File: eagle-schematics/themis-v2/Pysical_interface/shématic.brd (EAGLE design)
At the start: 160 x 100 mm, 35 parts, among them IC1 MCP23017SO, SW1 EC12E_SW, SW2 EC12E_SW, SW3 EC12E_SW, SW4 EC12E_SW

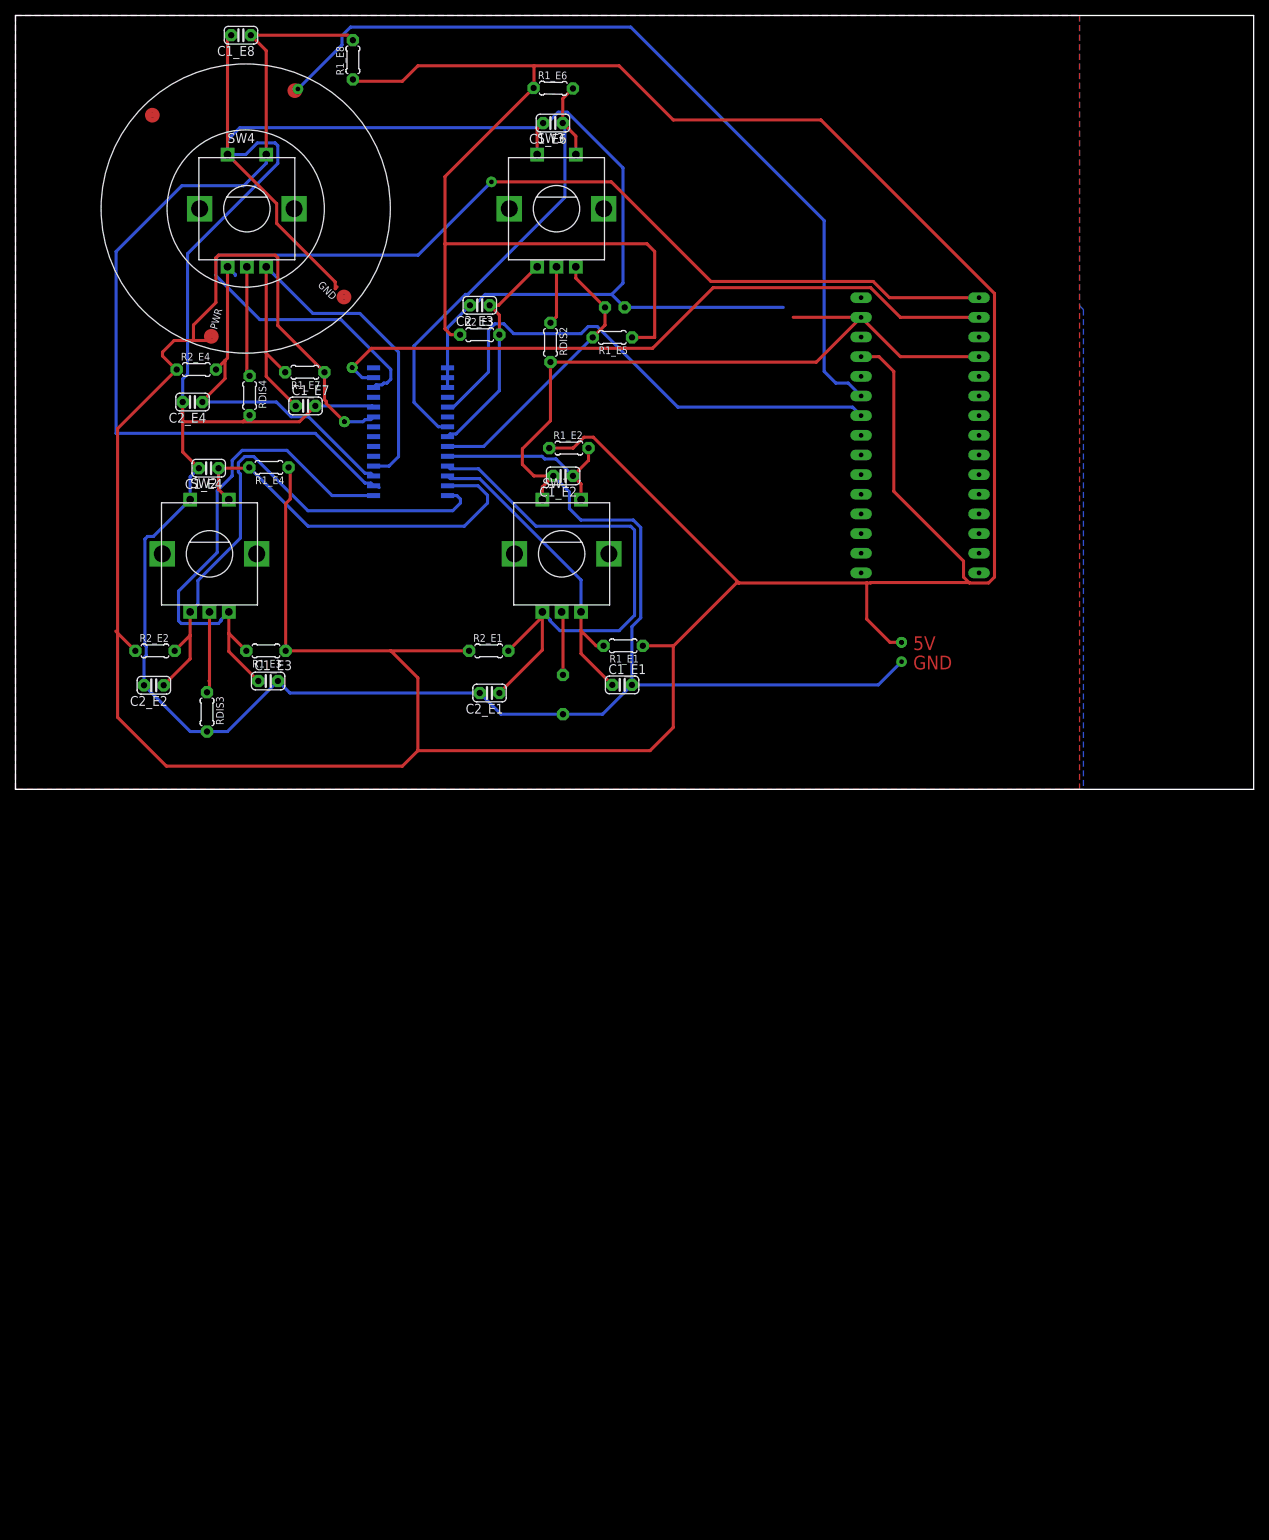
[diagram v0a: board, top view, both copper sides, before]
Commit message: Updated PCB
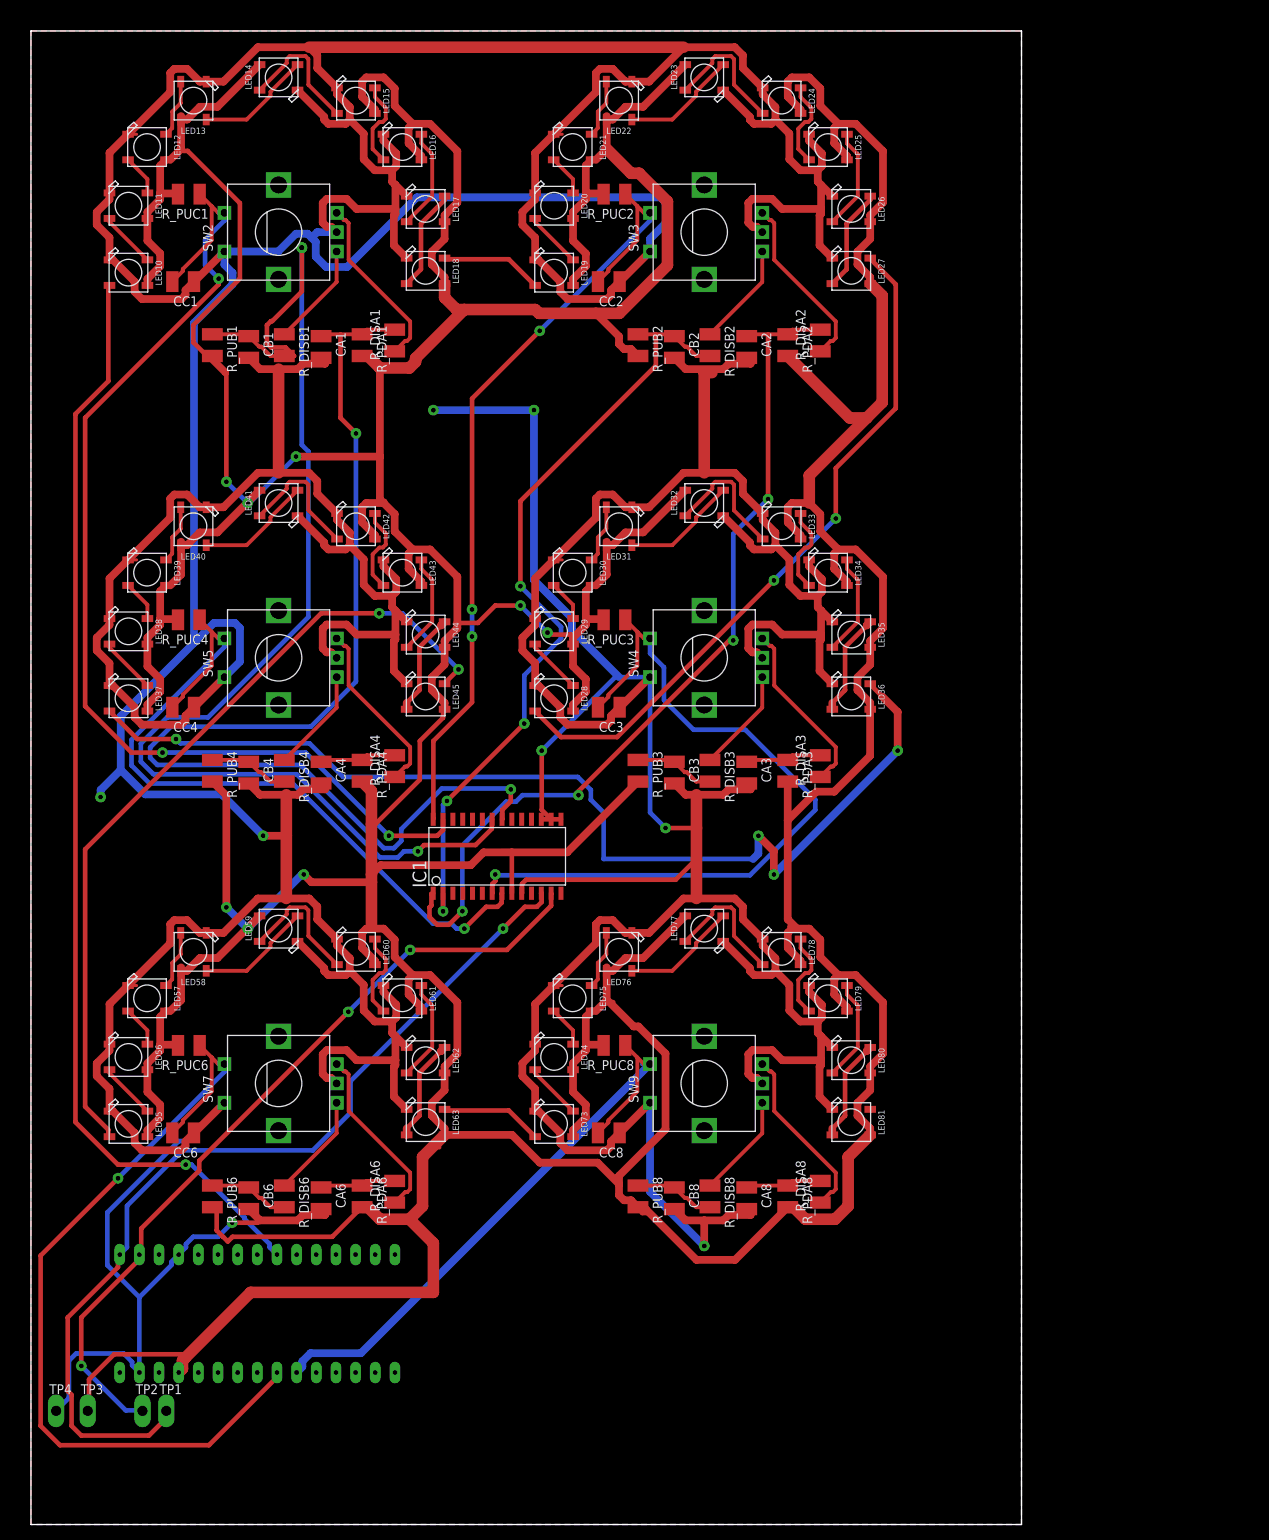
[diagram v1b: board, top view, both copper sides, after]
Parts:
- removed C1_E1, C1_E2, C1_E3, C1_E4, C1_E5, C1_E6, C1_E7, C1_E8, C2_E1, C2_E2, C2_E3, C2_E4: 100n, rcl:C025-024X044
- removed NEOPIXEL1: NEOPIXEL12, Neopixel:NEOPIXEL12
- removed R1_E1, R1_E2, R1_E3, R1_E4, R1_E5, R1_E6, R1_E7, R1_E8, R2_E1, R2_E2, R2_E3, R2_E4: 100k, resistor:0204/5
- removed RDIS1, RDIS2, RDIS3, RDIS4: 1k, resistor:0204/5
- removed SW1: EC12E_SW, switch-alps:ALPS_EC12E_SW
- added CA1, CA2, CA3, CA4, CA6, CA8, CB1, CB2, CB3, CB4, CB6, CB8, CC1, CC2, CC3, CC4, CC6, CC8: 100n, rcl:C1210
- added LED10, LED11, LED12, LED13, LED14, LED15, LED16, LED17, LED18, LED19, LED20, LED21, LED22, LED23, LED24, LED25, LED26, LED27, LED28, LED29, LED30, LED31, LED32, LED33, LED34, LED35, LED36, LED37, LED38, LED39, LED40, LED41, LED42, LED43, LED44, LED45, LED55, LED56, LED57, LED58, LED59, LED60, LED61, LED62, LED63, LED73, LED74, LED75, LED76, LED77, LED78, LED79, LED80, LED81: WS2812B5050, WS2812B:WS2812B
- added R_DISA1, R_DISA2, R_DISA3, R_DISA4, R_DISA6, R_DISA8, R_DISB1, R_DISB2, R_DISB3, R_DISB4, R_DISB6, R_DISB8: 1k, rcl:R1210
- added R_PDA1, R_PDA2, R_PDA3, R_PDA4, R_PDA6, R_PDA8, R_PUB1, R_PUB2, R_PUB3, R_PUB4, R_PUB6, R_PUB8, R_PUC1, R_PUC2, R_PUC3, R_PUC4, R_PUC6, R_PUC8: 100k, rcl:R1210
- added SW5, SW7, SW9: EC12E_SW, switch-alps:ALPS_EC12E_SW
- added TP1, TP2, TP3, TP4: PTR1PAD1-13Y, testpad:P1-13Y
- moved U$2 144.1 mm to (31.2, -75.4), turned to 0 degrees
- moved SW4 82.8 mm to (89.0, 17.0), turned to 90 degrees
- moved IC1 55.2 mm to (61.6, -8.65), flipped to the top, turned to 0 degrees
- moved SW2 42.5 mm to (34.0, 72.0), turned to 90 degrees
- moved SW3 19.3 mm to (89.0, 72.0), turned to 90 degrees
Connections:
- net INTA renamed INTROT_2
- net N$3 renamed INTROT1
- removed net BOUT_1: C1_E6.1, IC1.21, R1_E6.2, SW3.E
- removed net BOUT_2: C1_E2.1, IC1.24, R1_E2.2, SW1.E
- removed net BOUT_3: C1_E4.1, IC1.27, R1_E4.2, SW2.E
- removed net BOUT_4: C1_E8.1, IC1.2, R1_E8.2, SW4.E
- removed net DISCHARGE: RDIS1.1, RDIS2.1, RDIS3.1, RDIS4.1, SW1.C, SW2.C, SW3.C, SW4.C
- removed net EC1_1: C2_E3.1, IC1.22, R2_E3.2, SW3.A
- removed net EC1_2: C1_E5.1, IC1.23, R1_E5.2, SW3.B
- removed net EC2_1: C2_E1.1, IC1.25, R2_E1.2, SW1.A
- removed net EC2_2: C1_E1.1, IC1.26, R1_E1.2, SW1.B
- removed net EC3_1: C2_E2.1, IC1.28, R2_E2.2, SW2.A
- removed net EC3_2: C1_E3.1, IC1.1, R1_E3.2, SW2.B
- removed net EC4_1: C2_E4.1, IC1.3, R2_E4.2, SW4.A
- removed net EC4_2: C1_E7.1, IC1.4, R1_E7.2, SW4.B
- removed net INTB: IC1.19, U$2.A5
- removed net SPI1_DATA: NEOPIXEL1.P$IN, U$2.A6
- new net CLICK_1: CC1.2, IC1.27, R_PUC1.1, SW2.E
- new net CLICK_2: CC2.2, IC1.28, R_PUC2.1, SW3.E
- new net CLICK_3: CC3.2, IC1.7, R_PUC3.1, SW4.E
- new net CLICK_4: CC4.2, IC1.8, R_PUC4.1, SW5.E
- new net CLICK_5: CC6.2, R_PUC6.1, SW7.E, U$2.A3
- new net CLICK_6: CC8.2, R_PUC8.1, SW9.E, U$2.A2
- new net INTROT2: IC1.19
- new net INTROT_1: U$2.A5
- new net N$11: LED11.2-DOUT, LED12.4-DIN
- new net N$12: LED12.2-DOUT, LED13.4-DIN
- new net N$13: LED13.2-DOUT, LED14.4-DIN
- new net N$16: R_DISB1.1, SW2.A
- new net N$17: R_DISA1.1, SW2.B
- new net N$18: LED17.2-DOUT, LED18.4-DIN
- new net N$19: LED16.2-DOUT, LED17.4-DIN
- new net N$20: LED15.2-DOUT, LED16.4-DIN
- new net N$21: LED14.2-DOUT, LED15.4-DIN
- new net N$22: LED19.2-DOUT, LED20.4-DIN
- new net N$23: LED20.2-DOUT, LED21.4-DIN
- new net N$24: LED21.2-DOUT, LED22.4-DIN
- new net N$25: LED22.2-DOUT, LED23.4-DIN
- new net N$26: R_DISB2.1, SW3.A
- new net N$27: R_DISA2.1, SW3.B
- new net N$28: LED26.2-DOUT, LED27.4-DIN
- new net N$29: LED25.2-DOUT, LED26.4-DIN
- new net N$3: U$2.A1
- new net N$30: LED24.2-DOUT, LED25.4-DIN
- new net N$31: LED23.2-DOUT, LED24.4-DIN
- new net N$32: LED28.2-DOUT, LED29.4-DIN
- new net N$33: LED29.2-DOUT, LED30.4-DIN
- new net N$34: LED30.2-DOUT, LED31.4-DIN
- new net N$35: LED31.2-DOUT, LED32.4-DIN
- new net N$36: R_DISB3.1, SW4.A
- new net N$37: R_DISA3.1, SW4.B
- new net N$38: LED35.2-DOUT, LED36.4-DIN
- new net N$39: LED34.2-DOUT, LED35.4-DIN
- new net N$40: LED33.2-DOUT, LED34.4-DIN
- new net N$41: LED32.2-DOUT, LED33.4-DIN
- new net N$42: LED37.2-DOUT, LED38.4-DIN
- new net N$43: LED38.2-DOUT, LED39.4-DIN
- new net N$44: LED39.2-DOUT, LED40.4-DIN
- new net N$45: LED40.2-DOUT, LED41.4-DIN
- new net N$46: R_DISB4.1, SW5.A
- new net N$47: R_DISA4.1, SW5.B
- new net N$48: LED44.2-DOUT, LED45.4-DIN
- new net N$49: LED43.2-DOUT, LED44.4-DIN
- new net N$50: LED42.2-DOUT, LED43.4-DIN
- new net N$51: LED41.2-DOUT, LED42.4-DIN
- new net N$6: LED10.2-DOUT, LED11.4-DIN
- new net N$62: LED55.2-DOUT, LED56.4-DIN
- new net N$63: LED56.2-DOUT, LED57.4-DIN
- new net N$64: LED57.2-DOUT, LED58.4-DIN
- new net N$65: LED58.2-DOUT, LED59.4-DIN
- new net N$66: R_DISB6.1, SW7.A
- new net N$67: R_DISA6.1, SW7.B
- new net N$68: LED62.2-DOUT, LED63.4-DIN
- new net N$69: LED61.2-DOUT, LED62.4-DIN
- new net N$70: LED60.2-DOUT, LED61.4-DIN
- new net N$71: LED59.2-DOUT, LED60.4-DIN
- new net N$82: LED73.2-DOUT, LED74.4-DIN
- new net N$83: LED74.2-DOUT, LED75.4-DIN
- new net N$84: LED75.2-DOUT, LED76.4-DIN
- new net N$85: LED76.2-DOUT, LED77.4-DIN
- new net N$86: R_DISB8.1, SW9.A
- new net N$87: R_DISA8.1, SW9.B
- new net N$88: LED80.2-DOUT, LED81.4-DIN
- new net N$89: LED79.2-DOUT, LED80.4-DIN
- new net N$90: LED78.2-DOUT, LED79.4-DIN
- new net N$91: LED77.2-DOUT, LED78.4-DIN
- new net NEOPIXEL_IN: LED10.4-DIN, U$2.D6
- new net PIXEL_1: LED18.2-DOUT, LED19.4-DIN
- new net PIXEL_2: LED27.2-DOUT, LED28.4-DIN
- new net PIXEL_3: LED36.2-DOUT, LED37.4-DIN
- new net PIXEL_4: LED45.2-DOUT, LED55.4-DIN
- new net PIXEL_5: LED63.2-DOUT, LED73.4-DIN
- new net PIXEL_OUT: LED81.2-DOUT
- new net ROT1_1: CA1.1, IC1.21, R_DISA1.2, R_PDA1.1
- new net ROT1_2: CA2.1, IC1.1, R_DISA2.2, R_PDA2.1
- new net ROT1_3: CA3.1, R_DISA3.2, R_PDA3.1
- new net ROT1_4: CA4.1, R_DISA4.2, R_PDA4.1
- new net ROT1_5: CA6.1, R_DISA6.2, R_PDA6.1
- new net ROT1_6: CA8.1, R_DISA8.2, R_PDA8.1
- new net ROT2_1: CB1.1, IC1.22, R_DISB1.2, R_PUB1.1
- new net ROT2_2: CB2.1, IC1.2, R_DISB2.2, R_PUB2.1
- new net ROT2_3: CB3.1, R_DISB3.2, R_PUB3.1
- new net ROT2_4: CB4.1, R_DISB4.2, R_PUB4.1
- new net ROT2_5: CB6.1, R_DISB6.2, R_PUB6.1
- new net ROT2_6: CB8.1, R_DISB8.2, R_PUB8.1
- new net ROT3_1: IC1.23
- new net ROT3_2: IC1.3
- new net ROT4_1: IC1.24
- new net ROT4_2: IC1.4
- new net ROT5_1: IC1.25
- new net ROT5_2: IC1.5
- new net ROT6_1: IC1.26
- new net ROT6_2: IC1.6
- net GND: now also CA1.2, CA2.2, CA3.2, CA4.2, CA6.2, CA8.2, CB1.2, CB2.2, CB3.2, CB4.2, CB6.2, CB8.2, CC1.1, CC2.1, CC3.1, CC4.1, CC6.1, CC8.1, LED10.3-GND, LED11.3-GND, LED12.3-GND, LED13.3-GND, LED14.3-GND, LED15.3-GND, LED16.3-GND, LED17.3-GND, LED18.3-GND, LED19.3-GND, LED20.3-GND, LED21.3-GND, LED22.3-GND, LED23.3-GND, LED24.3-GND, LED25.3-GND, LED26.3-GND, LED27.3-GND, LED28.3-GND, LED29.3-GND, LED30.3-GND, LED31.3-GND, LED32.3-GND, LED33.3-GND, LED34.3-GND, LED35.3-GND, LED36.3-GND, LED37.3-GND, LED38.3-GND, LED39.3-GND, LED40.3-GND, LED41.3-GND, LED42.3-GND, LED43.3-GND, LED44.3-GND, LED45.3-GND, LED55.3-GND, LED56.3-GND, LED57.3-GND, LED58.3-GND, LED59.3-GND, LED60.3-GND, LED61.3-GND, LED62.3-GND, LED63.3-GND, LED73.3-GND, LED74.3-GND, LED75.3-GND, LED76.3-GND, LED77.3-GND, LED78.3-GND, LED79.3-GND, LED80.3-GND, LED81.3-GND, SW2.C, SW3.C, SW4.C, SW5.C, SW5.D, SW7.C, SW7.D, SW9.C, SW9.D, TP4.TP; no longer C1_E1.2, C1_E2.2, C1_E3.2, C1_E4.2, C1_E5.2, C1_E6.2, C1_E7.2, C1_E8.2, C2_E1.2, C2_E2.2, C2_E3.2, C2_E4.2, RDIS1.2, RDIS2.2, RDIS3.2, RDIS4.2, SW1.D
- net I2C_CLK: now also TP1.TP
- net I2C_DATA: now also TP2.TP
- net VCC: now also LED10.1-VDD, LED11.1-VDD, LED12.1-VDD, LED13.1-VDD, LED14.1-VDD, LED15.1-VDD, LED16.1-VDD, LED17.1-VDD, LED18.1-VDD, LED19.1-VDD, LED20.1-VDD, LED21.1-VDD, LED22.1-VDD, LED23.1-VDD, LED24.1-VDD, LED25.1-VDD, LED26.1-VDD, LED27.1-VDD, LED28.1-VDD, LED29.1-VDD, LED30.1-VDD, LED31.1-VDD, LED32.1-VDD, LED33.1-VDD, LED34.1-VDD, LED35.1-VDD, LED36.1-VDD, LED37.1-VDD, LED38.1-VDD, LED39.1-VDD, LED40.1-VDD, LED41.1-VDD, LED42.1-VDD, LED43.1-VDD, LED44.1-VDD, LED45.1-VDD, LED55.1-VDD, LED56.1-VDD, LED57.1-VDD, LED58.1-VDD, LED59.1-VDD, LED60.1-VDD, LED61.1-VDD, LED62.1-VDD, LED63.1-VDD, LED73.1-VDD, LED74.1-VDD, LED75.1-VDD, LED76.1-VDD, LED77.1-VDD, LED78.1-VDD, LED79.1-VDD, LED80.1-VDD, LED81.1-VDD, R_PDA1.2, R_PDA2.2, R_PDA3.2, R_PDA4.2, R_PDA6.2, R_PDA8.2, R_PUB1.2, R_PUB2.2, R_PUB3.2, R_PUB4.2, R_PUB6.2, R_PUB8.2, R_PUC1.2, R_PUC2.2, R_PUC3.2, R_PUC4.2, R_PUC6.2, R_PUC8.2, TP3.TP; no longer NEOPIXEL1.P$5V, R1_E1.1, R1_E2.1, R1_E3.1, R1_E4.1, R1_E5.1, R1_E6.1, R1_E7.1, R1_E8.1, R2_E1.1, R2_E2.1, R2_E3.1, R2_E4.1
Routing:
- net GND: track 522.6 -> 1427.9 mm, vias 1 -> 8
- net VCC: track 604.0 -> 1159.7 mm, vias 4 -> 8
- net ROT2_1: track 0.00 -> 162.3 mm, vias 0 -> 3
- net ROT1_1: track 0.00 -> 148.1 mm, vias 0 -> 2
- net NEOPIXEL_IN: track 0.00 -> 144.7 mm, vias 0 -> 1
- net CLICK_1: track 0.00 -> 143.6 mm, vias 0 -> 3
- net PIXEL_3: track 0.00 -> 137.5 mm, vias 0 -> 4
- net ROT1_2: track 0.00 -> 115.9 mm, vias 0 -> 4
- net BOUT_4: track 115.4 -> 0.00 mm
- net CLICK_5: track 0.00 -> 108.4 mm, vias 0 -> 1
- net SPI1_DATA: track 108.4 -> 0.00 mm, vias 1 -> 0
- net CLICK_2: track 0.00 -> 106.0 mm, vias 0 -> 3
- net PIXEL_4: track 0.00 -> 104.9 mm, vias 0 -> 2
- net ROT2_2: track 0.00 -> 103.1 mm, vias 0 -> 4
- net CLICK_3: track 0.00 -> 98.5 mm, vias 0 -> 1
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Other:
- board size 160 x 100 mm -> 128 x 193 mm
- board text removed: "5V"
- board text removed: "GND"
